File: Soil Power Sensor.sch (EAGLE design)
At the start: 61 parts, among them U1 ADS1219IRTER, U11 ESP32-C3-MINI-1-N4, U2 INA296A5, U3 THS4532, U4 TPS60400DBV, U6 REF2033, U7 WIO-E5_MINI, U9 MAX9944ASA, X1 Voltage, X2 Current, X3 GND, X4 SDI

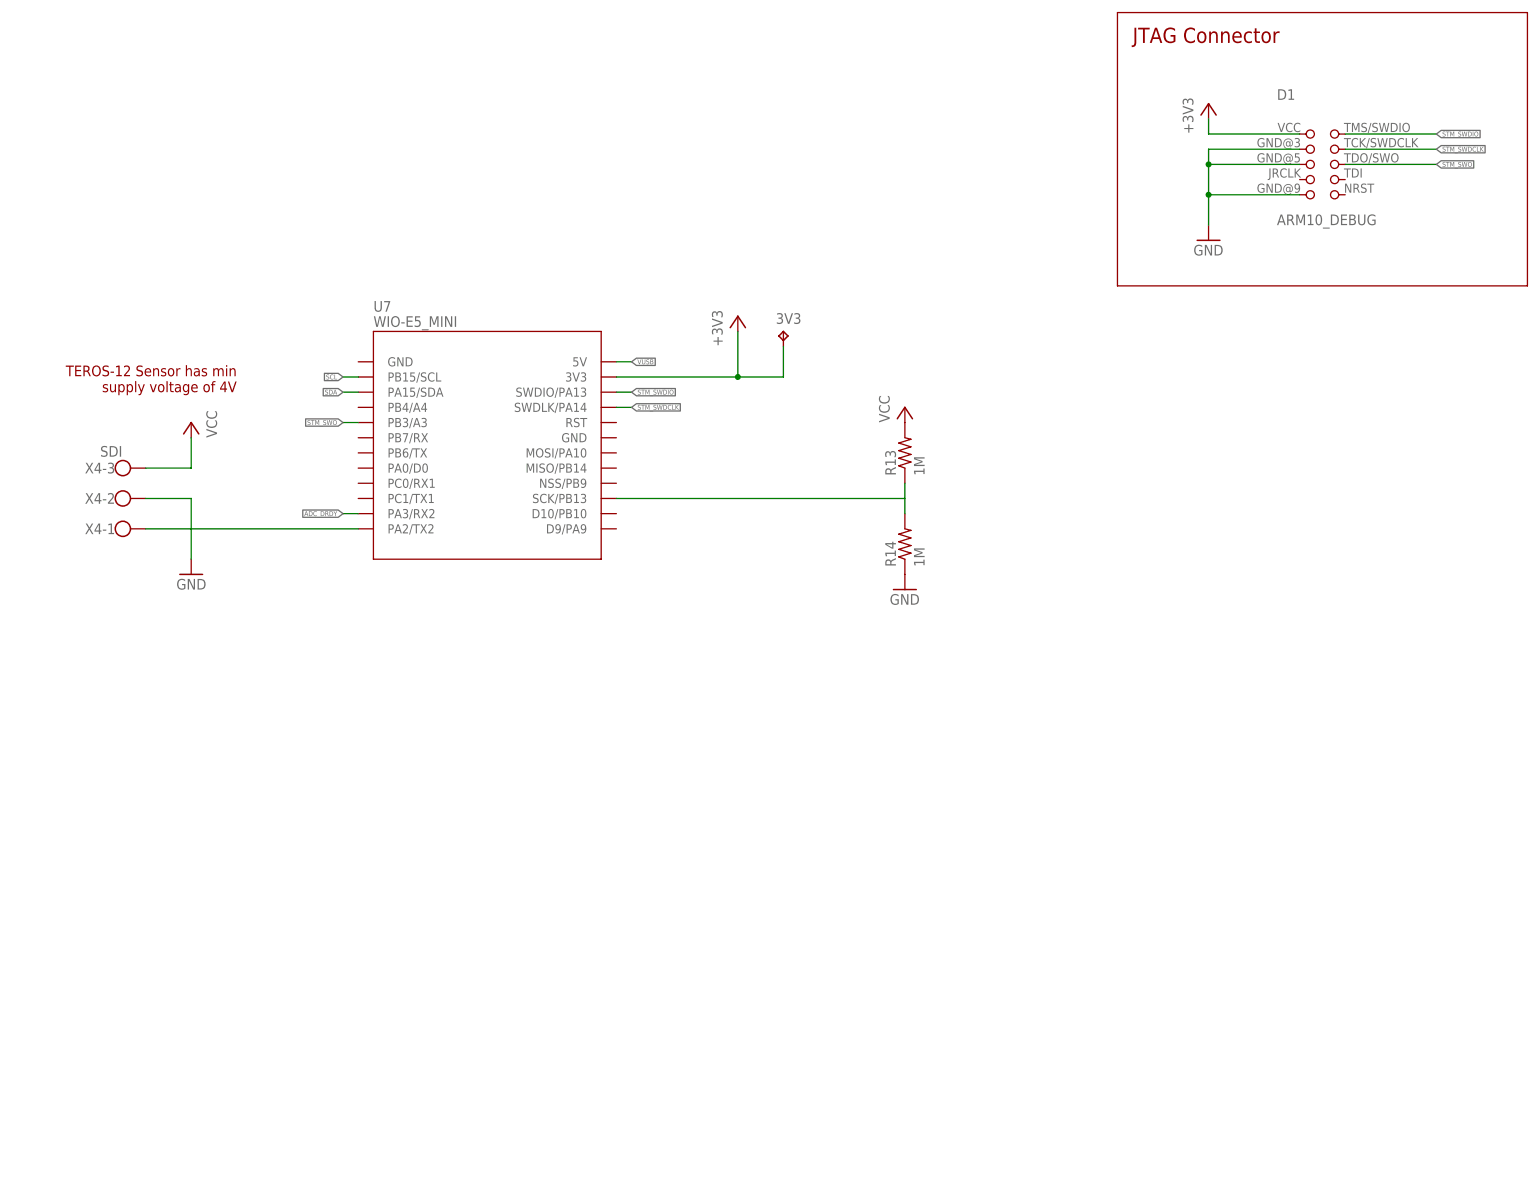
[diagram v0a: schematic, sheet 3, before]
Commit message: Closes #9
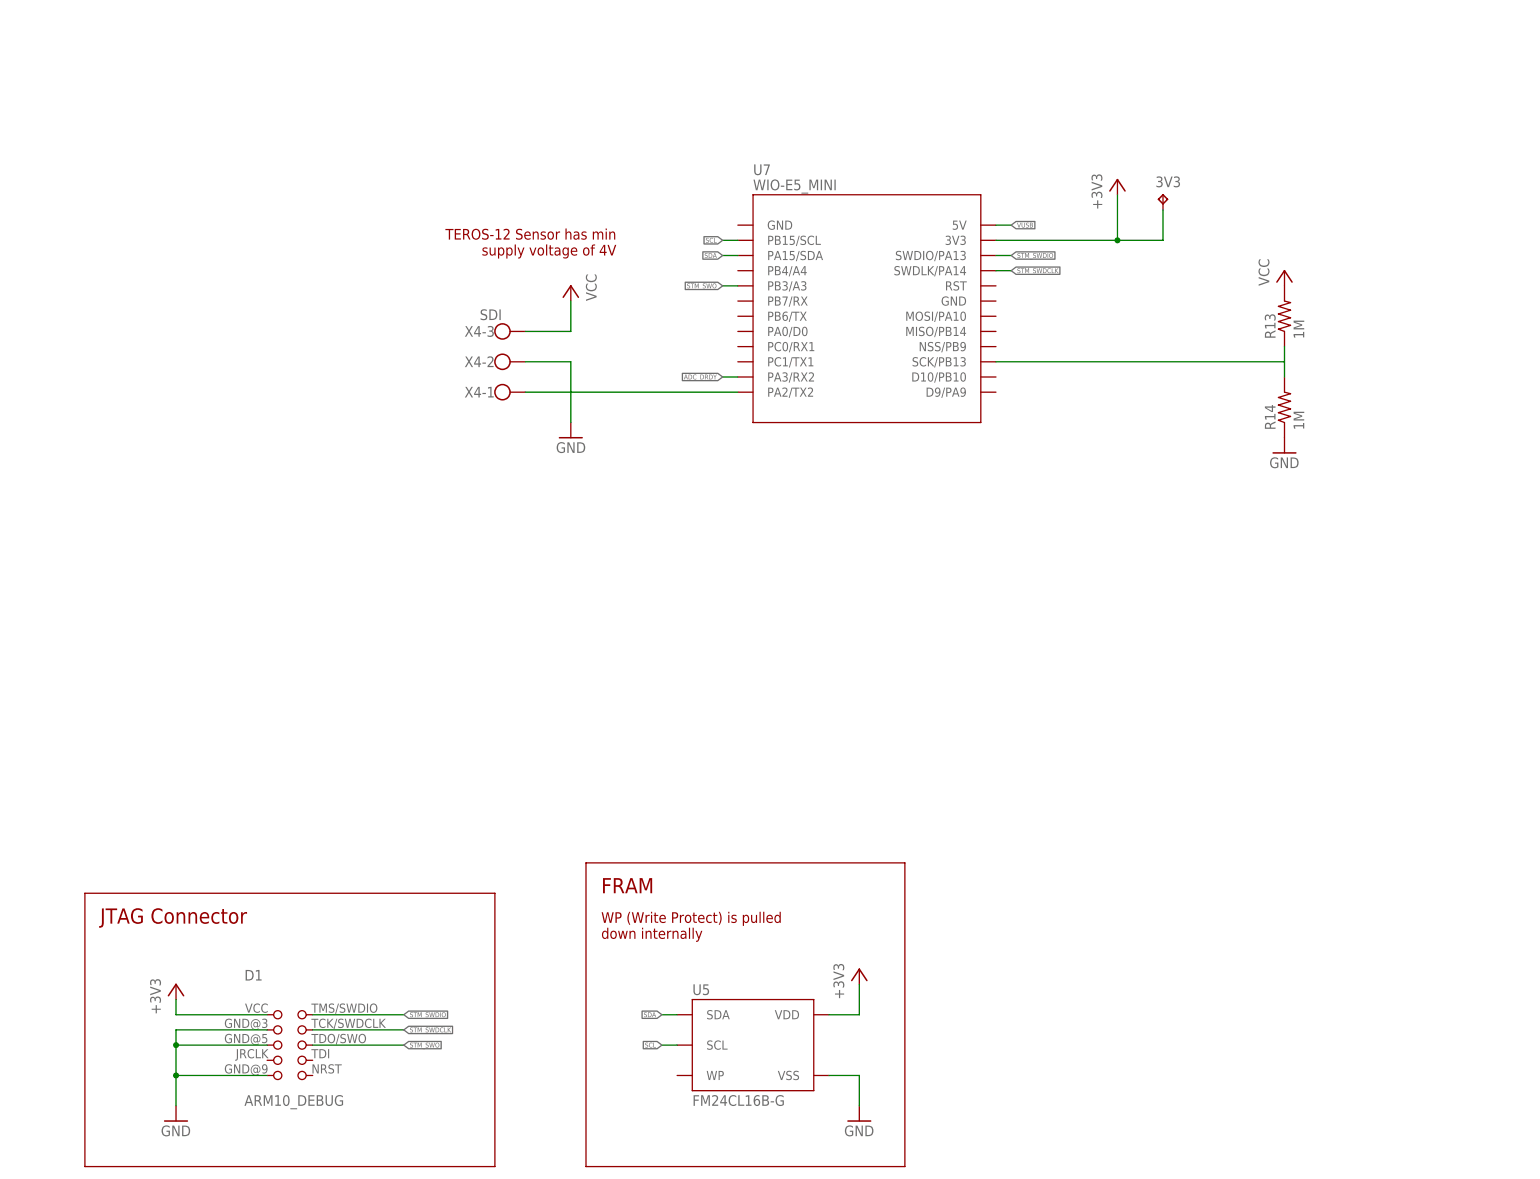
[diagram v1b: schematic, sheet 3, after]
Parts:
- added U5: FM24CL16B-G, Soil Power Sensor:FM24CL16B-G
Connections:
- net +3V3: now also U5.VDD
- net GND: now also U5.VSS
- net SCL: now also U5.SCL
- net SDA: now also U5.SDA
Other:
- note added: "FRAM"
- note added: "WP (Write Protect) is pulled down internally"
- moved on the sheet: 3V3, D1, R13, R14, U7, X4-1, X4-2, X4-3
